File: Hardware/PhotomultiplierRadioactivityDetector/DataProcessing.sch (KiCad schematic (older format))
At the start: 36 parts, among them J1 Conn_01x04_Female, J2 Conn_01x04_Female, U5 STM32F030K6Tx, Y1 20MHz

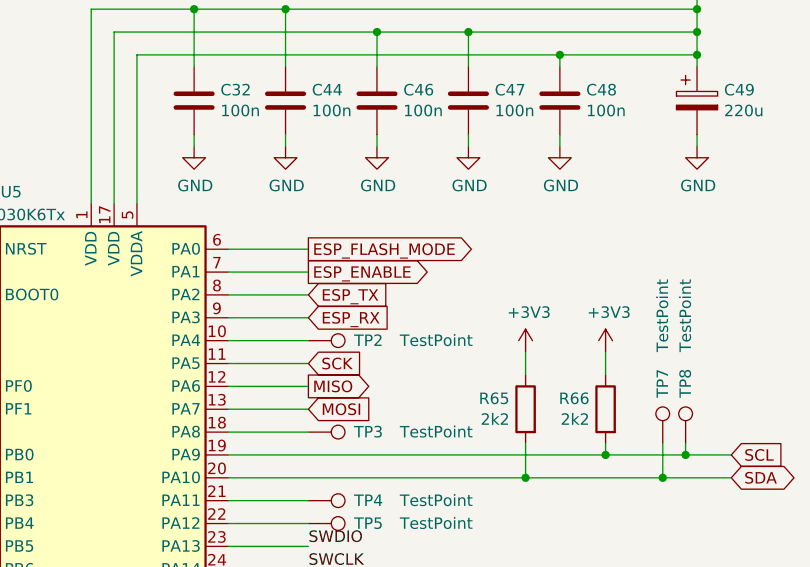
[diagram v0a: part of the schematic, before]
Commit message: placement of components for hw generator
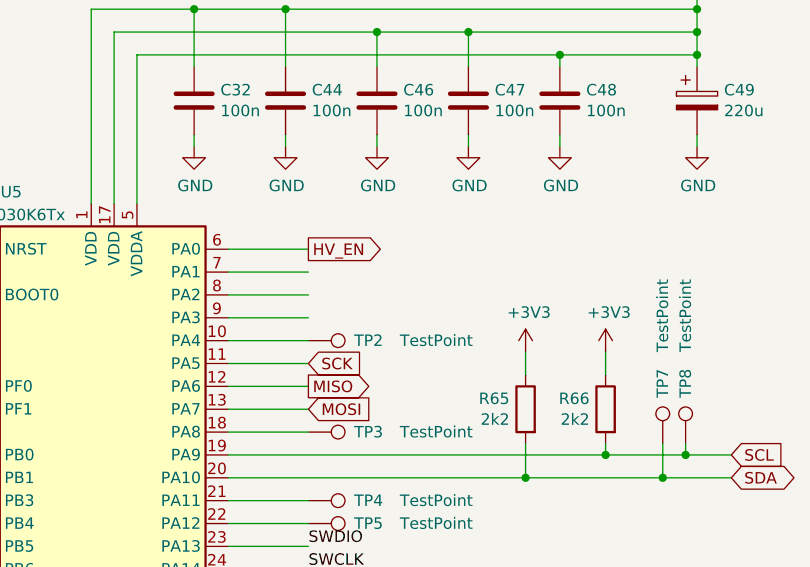
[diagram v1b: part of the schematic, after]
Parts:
- D6, D7, D8: footprint LED_SMD:LED_0402_1005Metric -> LED_SMD:LED_0805_2012Metric
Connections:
- net labels added: HV_EN
- net labels removed: ESP_ENABLE, ESP_FLASH_MODE, ESP_RX, ESP_TX
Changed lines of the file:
@@
 Wire Wire Line
 	2400 3050 2400 3100
-Text GLabel 4550 3250 2    50   Output ~ 0
-ESP_ENABLE
-Text GLabel 4550 3150 2    50   Output ~ 0
-ESP_FLASH_MODE
-Text GLabel 4550 3350 2    50   Input ~ 0
-ESP_TX
-Text GLabel 4550 3450 2    50   Input ~ 0
-ESP_RX
 Text GLabel 2700 4150 0    50   Output ~ 0
 CS_ESP
@@
 F 0 "D6" V 1589 4733 50  0000 R CNN
 F 1 "LED" V 1498 4733 50  0000 R CNN
-F 2 "LED_SMD:LED_0402_1005Metric" H 1550 4850 50  0001 C CNN
+F 2 "LED_SMD:LED_0805_2012Metric" H 1550 4850 50  0001 C CNN
 F 3 "~" H 1550 4850 50  0001 C CNN
 	1    1550 4850
@@
 F 0 "D7" V 1939 4733 50  0000 R CNN
 F 1 "LED" V 1848 4733 50  0000 R CNN
-F 2 "LED_SMD:LED_0402_1005Metric" H 1900 4850 50  0001 C CNN
+F 2 "LED_SMD:LED_0805_2012Metric" H 1900 4850 50  0001 C CNN
 F 3 "~" H 1900 4850 50  0001 C CNN
 	1    1900 4850
@@
 F 0 "D8" V 2289 4733 50  0000 R CNN
 F 1 "LED" V 2198 4733 50  0000 R CNN
-F 2 "LED_SMD:LED_0402_1005Metric" H 2250 4850 50  0001 C CNN
+F 2 "LED_SMD:LED_0805_2012Metric" H 2250 4850 50  0001 C CNN
 F 3 "~" H 2250 4850 50  0001 C CNN
 	1    2250 4850
@@
 	1    0    0    -1
 $EndComp
+Text GLabel 4550 3150 2    50   Output ~ 0
+HV_EN
 $EndSCHEMATC
